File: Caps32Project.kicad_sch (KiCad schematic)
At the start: 23 parts, among them J1 Ph 2.0, J2 Sh 1.0, P1 USB_C_Plug_USB2.0, Q1 AO3401A, U1 MPU-6050, U2 MAX17048G_T10, U3 ESP32C3_SuperMini, U4 MCP73831-2-OT

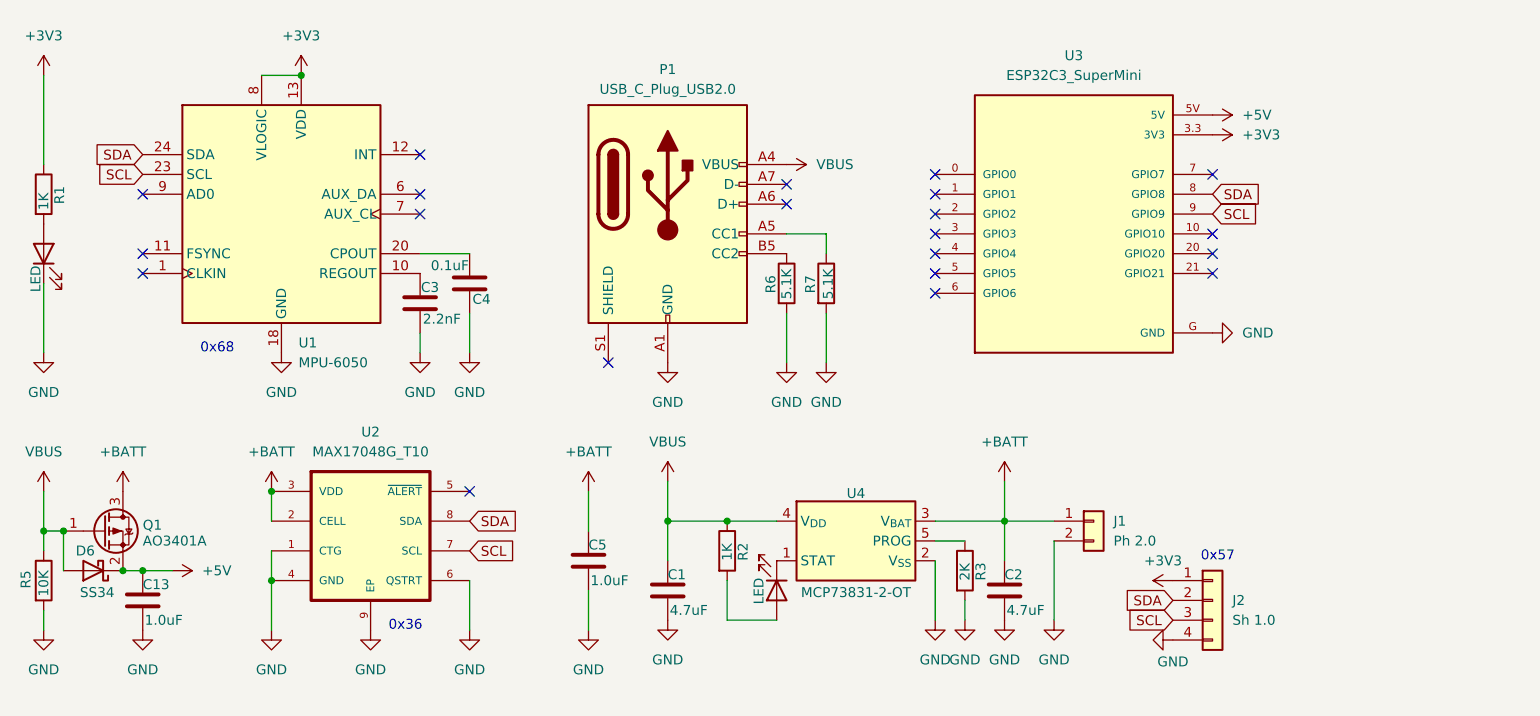
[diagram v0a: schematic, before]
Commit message: LGTM
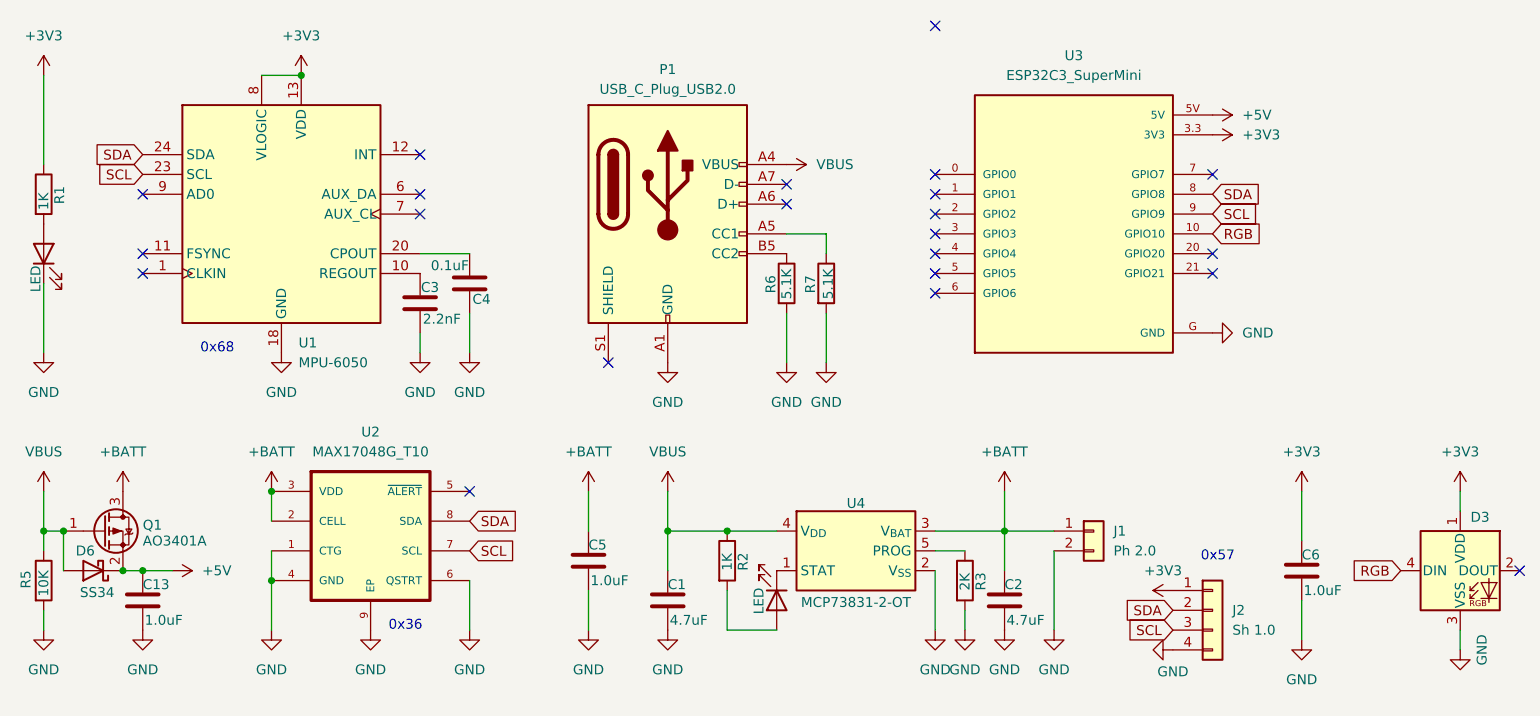
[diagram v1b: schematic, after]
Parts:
- added C6: 1.0uF, Capacitor_SMD:C_0402_1005Metric_Pad0.74x0.62mm_HandSolder, symbol Device:C
- added D3: WS2812B, LED_SMD:LED_WS2812B_PLCC4_5.0x5.0mm_P3.2mm, symbol LED:WS2812B
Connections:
- net +3V3: now also C6.1, D3.1 (VDD)
- net GND: now also C6.2, D3.3 (VSS)
- net RGB: now reaches U3.10 (GPIO10)
- net RGB: now also D3.4 (DIN)
- no-connect marks 21 -> 22
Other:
- moved on the sheet: C1, C2, J1, J2, R2, R3, U4

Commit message: MH42
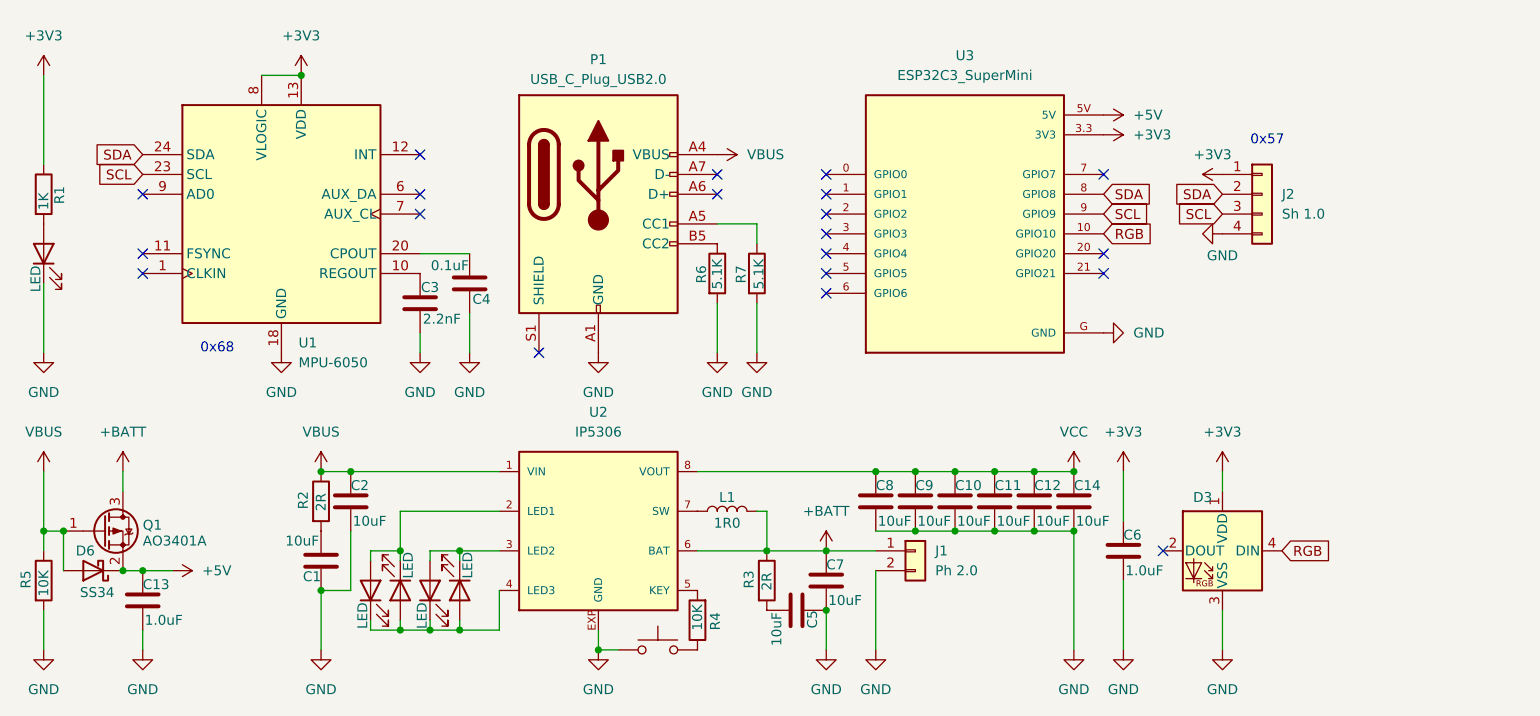
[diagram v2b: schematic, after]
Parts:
- removed U2: MAX17048G_T10, Custom:SON50P200X200X80-9N, symbol Custom:MAX17048G_T10
- removed U4: MCP73831-2-OT, Package_TO_SOT_SMD:SOT-23-5, symbol Battery_Management:MCP73831-5-OT
- added C10, C11, C12, C14, C7, C8, C9: 10uF, Capacitor_SMD:C_0402_1005Metric_Pad0.74x0.62mm_HandSolder, symbol Device:C
- added D4, D5, D7: LED, LED_SMD:LED_0402_1005Metric_Pad0.77x0.64mm_HandSolder, symbol Device:LED
- added L1: 1R0, symbol Device:L
- added R4: 10K, Resistor_SMD:R_0402_1005Metric_Pad0.72x0.64mm_HandSolder, symbol Device:R
- added SW1: SW_Push, symbol Switch:SW_Push
- added U2: IP5306, IP5306:SOP8-P, symbol Custom:IP5306
- C1, C2: value 4.7uF -> 10uF
- C5: value 1.0uF -> 10uF
- R2: value 1K -> 2R
- R3: value 2K -> 2R
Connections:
- net +BATT: now also R3.1, C7.1, L1.2, U2.6 (BAT); no longer C2.1, C5.1
- net GND: now also C1.1, C5.1, C10.2, C11.2, C12.2, C14.2, C7.2, C8.2, C9.2, SW1.1, U2.EXP (GND); no longer C1.2, C5.2, R3.2
- net VBUS: now also C2.1, U2.1 (VIN); no longer C1.1
- net at D2.2 (A): now also D4.1 (K), U2.2 (LED1); no longer R2.2
- net at D2.1 (K): now also D4.2 (A), D5.1 (K), D7.2 (A), U2.4 (LED3)
- new net: D5.2 (A), D7.1 (K), U2.3 (LED2)
- new net: C1.2, R2.2
- new net: C5.2, R3.2
- new net: R4.1, SW1.2
- new net: R4.2, U2.5 (KEY)
- new net: L1.1, U2.7 (SW)
- new net VCC: C10.1, C11.1, C12.1, C14.1, C8.1, C9.1, U2.8 (VOUT)
- no-connect marks 22 -> 20
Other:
- moved on the sheet: C6, D3, J1, J2, P1, R6, R7, U3

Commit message: Tweak
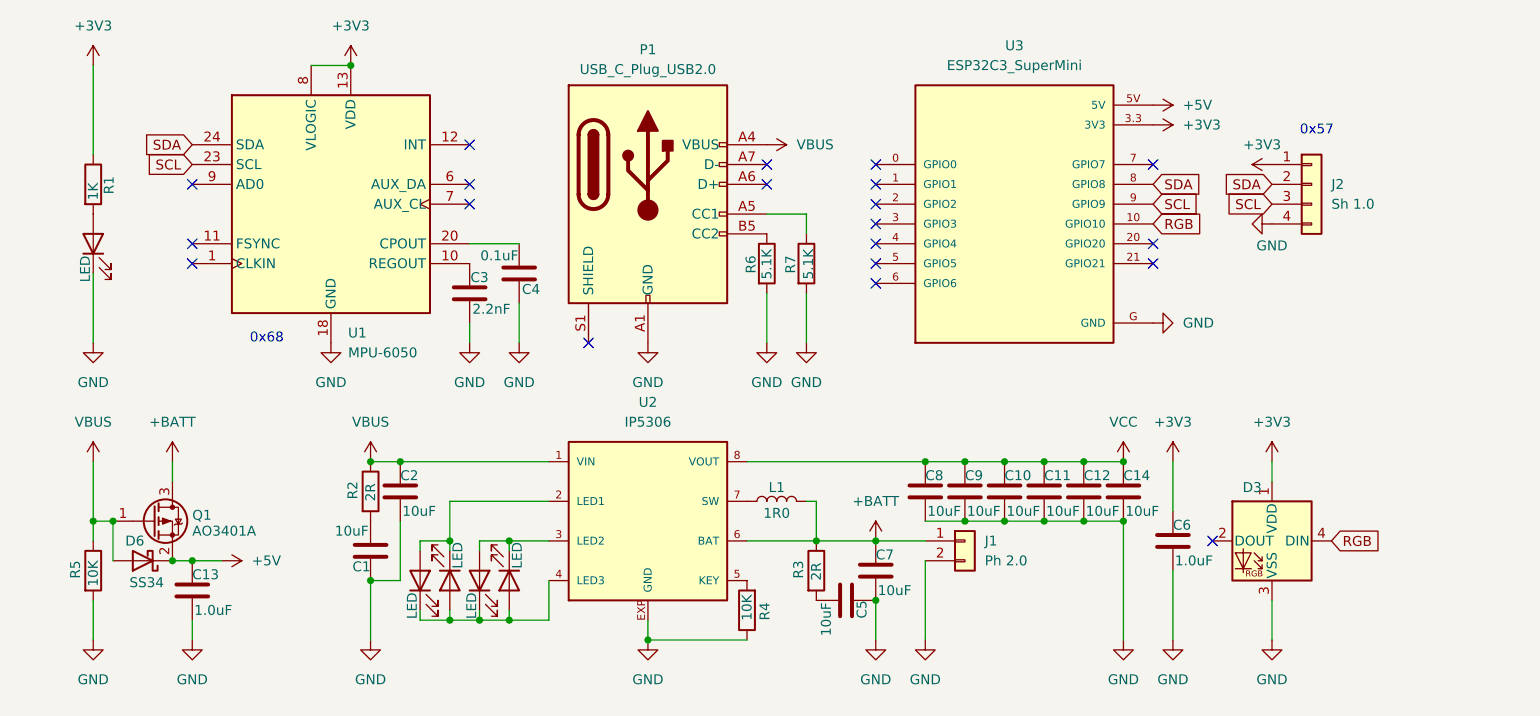
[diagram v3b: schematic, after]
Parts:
- removed SW1: SW_Push, symbol Switch:SW_Push
- L1: footprint (none) -> Inductor_SMD:L_6.3x6.3_H3
- P1: footprint Connector_USB:USB_C_Receptacle_XKB_U262-16XN-4BVC11 -> Connector_USB:USB_C_Receptacle_Palconn_UTC16-G
- U2: footprint IP5306:SOP8-P -> Custom:IP5306
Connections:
- net GND: now also R4.1
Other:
- moved on the sheet: C1, C10, C11, C12, C13, C14, C2, C3, C4, C5, C6, C7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

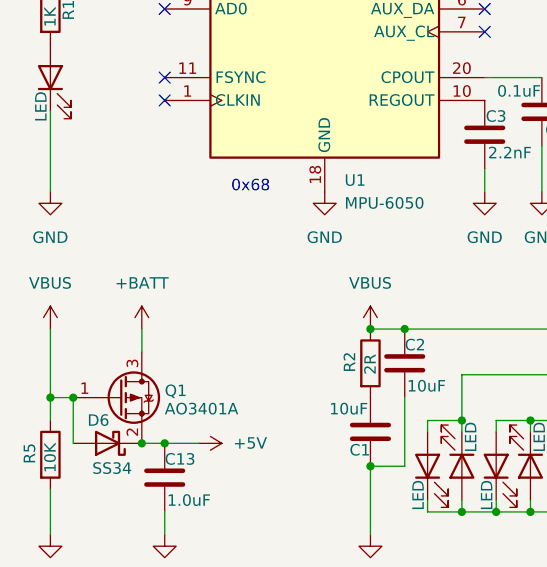
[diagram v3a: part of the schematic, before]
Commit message: Non Latch
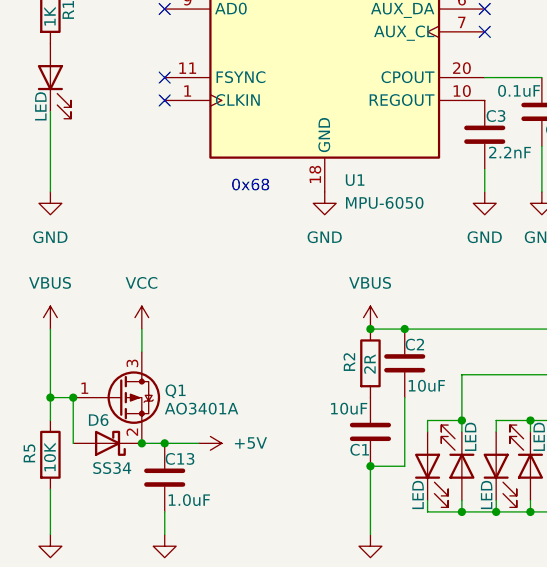
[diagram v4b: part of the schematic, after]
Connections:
- net +BATT: no longer Q1.3 (D)
- net VCC: now also Q1.3 (D)
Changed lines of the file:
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@@
+	)
+	(symbol
+		(lib_id "power:VCC")
+		(at 36.83 72.39 0)
+		(unit 1)
+		(exclude_from_sim no)
+		(in_bom yes)
+		(on_board yes)
+		(dnp no)
+		(fields_autoplaced yes)
+		(property "Reference" "#PWR022"
+			(at 36.83 76.2 0)
+			(effects
+				(font
+					(size 1.27 1.27)
+				)
+				(hide yes)
+			)
+		)
+		(property "Value" "VCC"
+			(at 36.83 67.31 0)
+			(effects
+				(font
+					(size 1.27 1.27)
+				)
+			)
+		)
+		(property "Footprint" ""
+			(at 36.83 72.39 0)
+			(effects
+				(font
+					(size 1.27 1.27)
+				)
+				(hide yes)
+			)
+		)
+		(property "Datasheet" ""
+			(at 36.83 72.39 0)
+			(effects
+				(font
+					(size 1.27 1.27)
+				)
+				(hide yes)
+			)
+		)
+		(property "Description" "Power symbol creates a global label with name \"VCC\""
+			(at 36.83 72.39 0)
+			(effects
+				(font
+					(size 1.27 1.27)
+				)
+				(hide yes)
+			)
+		)
+		(pin "1"
+		)
+		(instances
+			(project "Caps32Project"
+				(path "/c1972a26-8b03-42e6-af88-e08ef9733d83"
+					(reference "#PWR022")
+					(unit 1)
+				)
+			)
+		)
 	)
 	(symbol
@@
 					(unit 1)
 				)
-			)
-		)
-	)
-	(symbol
-		(lib_id "power:+BATT")
-		(at 36.83 72.39 0)
-		(unit 1)
-		(exclude_from_sim no)
-		(in_bom yes)
-		(on_board yes)
-		(dnp no)
-		(fields_autoplaced yes)
-		(property "Reference" "#PWR022"
-			(at 36.83 76.2 0)
-			(effects
-				(font
-					(size 1.27 1.27)
-				)
-				(hide yes)
-			)
-		)
-		(property "Value" "+BATT"
-			(at 36.83 67.31 0)
-			(effects
-				(font
-					(size 1.27 1.27)
-				)
-			)
-		)
-		(property "Footprint" ""
-			(at 36.83 72.39 0)
-			(effects
-				(font
-					(size 1.27 1.27)
-				)
-				(hide yes)
-			)
-		)
-		(property "Datasheet" ""
-			(at 36.83 72.39 0)
-			(effects
-				(font
-					(size 1.27 1.27)
-				)
-				(hide yes)
-			)
-		)
-		(property "Description" "Power symbol creates a global label with name \"+BATT\""
-			(at 36.83 72.39 0)
-			(effects
-				(font
-					(size 1.27 1.27)
-				)
-				(hide yes)
-			)
-		)
-		(pin "1"
-		)
-		(instances
-			(project "Caps"
-				(path "/c1972a26-8b03-42e6-af88-e08ef9733d83"
-					(reference "#PWR022")
-					(unit 1)
-				)

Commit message: Tweak
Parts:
- U3: footprint Custom:ESP32C3_Supermini_THT -> Custom:Supermini_Custom
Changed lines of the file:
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@@
 			)
 		)
-		(property "Footprint" "Custom:ESP32C3_Supermini_THT"
+		(property "Footprint" "Custom:Supermini_Custom"
 			(at 144.78 39.37 0)
 			(effects

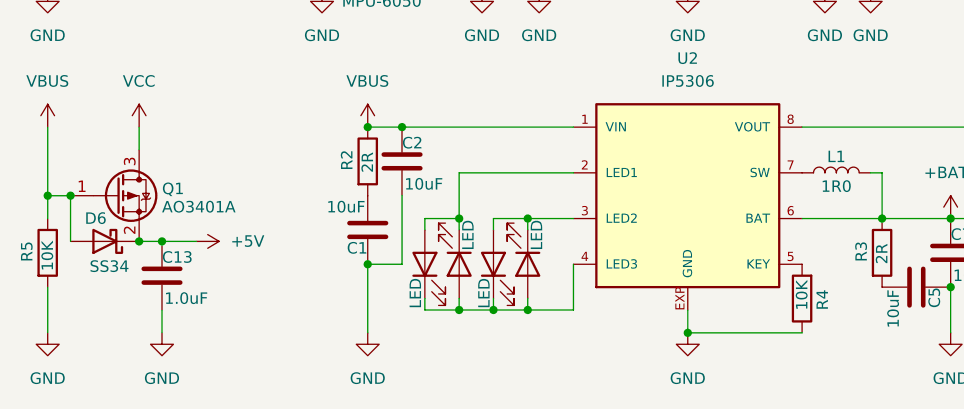
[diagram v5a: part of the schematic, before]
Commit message: Fixing
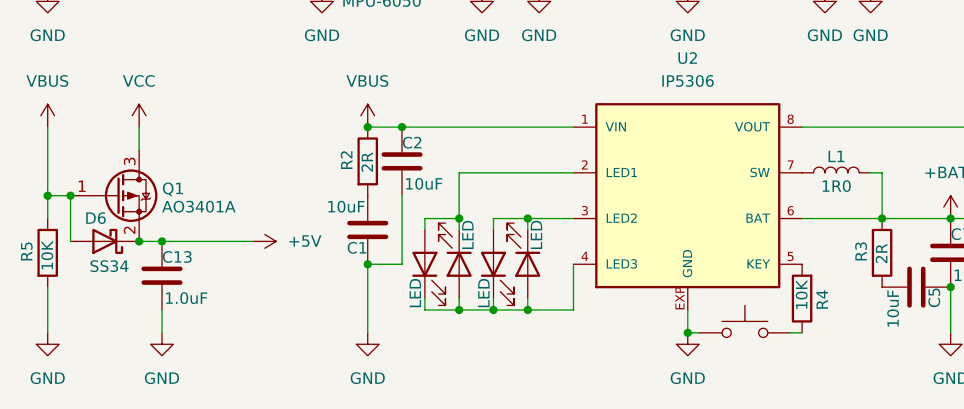
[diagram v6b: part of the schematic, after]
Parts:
- added SW1: SW_Push, Button_Switch_SMD:SW_Push_1TS009xxxx-xxxx-xxxx_6x6x5mm, symbol Switch:SW_Push
- J1: footprint Connector_JST:JST_PH_S2B-PH-K_1x02_P2.00mm_Horizontal -> Connector_JST:JST_PH_S2B-PH-SM4-TB_1x02-1MP_P2.00mm_Horizontal
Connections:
- net GND: now also SW1.1; no longer R4.1
- new net: R4.1, SW1.2
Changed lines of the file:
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@@
 	)
 	(junction
-		(at 97.79 95.25)
-		(diameter 0)
-		(color 0 0 0 0)
-	)
-	(junction
 		(at 127 90.17)
 		(diameter 0)
@@
 	)
 	(junction
+		(at 97.79 95.25)
+		(diameter 0)
+		(color 0 0 0 0)
+	)
+	(junction
 		(at 26.67 80.01)
 		(diameter 0)
@@
 	(wire
 		(pts
+			(xy 97.79 95.25) (xy 99.06 95.25)
+		)
+		(stroke
+			(width 0)
+			(type default)
+		)
+	)
+	(wire
+		(pts
 			(xy 118.11 40.64) (xy 113.03 40.64)
 		)
@@
 	(wire
 		(pts
-			(xy 97.79 95.25) (xy 110.49 95.25)
+			(xy 109.22 95.25) (xy 110.49 95.25)
 		)
 		(stroke
@@
 	(wire
 		(pts
-			(xy 43.18 85.09) (xy 39.37 85.09)
+			(xy 49.53 85.09) (xy 39.37 85.09)
 		)
 		(stroke
@@
 	(symbol
 		(lib_id "power:+5V")
-		(at 43.18 85.09 270)
+		(at 49.53 85.09 270)
 		(unit 1)
 		(exclude_from_sim no)
@@
 		(fields_autoplaced yes)
 		(property "Reference" "#PWR014"
-			(at 39.37 85.09 0)
+			(at 45.72 85.09 0)
 			(effects
 				(font
@@
 		)
 		(property "Value" "+5V"
-			(at 46.99 85.0899 90)
+			(at 53.34 85.0899 90)
 			(effects
 				(font
@@
 		)
 		(property "Footprint" ""
-			(at 43.18 85.09 0)
+			(at 49.53 85.09 0)
 			(effects
 				(font
@@
 		)
 		(property "Datasheet" ""
-			(at 43.18 85.09 0)
+			(at 49.53 85.09 0)
 			(effects
 				(font
@@
 		)
 		(property "Description" "Power symbol creates a global label with name \"+5V\""
-			(at 43.18 85.09 0)
+			(at 49.53 85.09 0)
 			(effects
 				(font
@@
 	)
 	(symbol
+		(lib_id "Switch:SW_Push")
+		(at 104.14 95.25 0)
+		(unit 1)
+		(exclude_from_sim no)
+		(in_bom yes)
+		(on_board yes)
+		(dnp no)
+		(fields_autoplaced yes)
+		(property "Reference" "SW1"
+			(at 104.14 87.63 0)
+			(effects
+				(font
+					(size 1.27 1.27)
+				)
+				(hide yes)
+			)
+		)
+		(property "Value" "SW_Push"
+			(at 104.14 90.17 0)
+			(effects
+				(font
+					(size 1.27 1.27)
+				)
+				(hide yes)
+			)
+		)
+		(property "Footprint" "Button_Switch_SMD:SW_Push_1TS009xxxx-xxxx-xxxx_6x6x5mm"
+			(at 104.14 90.17 0)
+			(effects
+				(font
+					(size 1.27 1.27)
+				)
+				(hide yes)
+			)
+		)
+		(property "Datasheet" "~"
+			(at 104.14 90.17 0)
+			(effects
+				(font
+					(size 1.27 1.27)
+				)
+				(hide yes)
+			)
+		)
+		(property "Description" "Push button switch, generic, two pins"
+			(at 104.14 95.25 0)
+			(effects
+				(font
+					(size 1.27 1.27)
+				)
+				(hide yes)
+			)
+		)
+		(pin "1"
+		)
+		(pin "2"
+		)
+		(instances
+			(project ""
+				(path "/c1972a26-8b03-42e6-af88-e08ef9733d83"
+					(reference "SW1")
+					(unit 1)
+				)
+			)
+		)
+	)
+	(symbol
 		(lib_id "Device:L")
 		(at 114.3 77.47 90)
@@
 			)
 		)
-		(property "Footprint" "Connector_JST:JST_PH_S2B-PH-K_1x02_P2.00mm_Horizontal"
+		(property "Footprint" "Connector_JST:JST_PH_S2B-PH-SM4-TB_1x02-1MP_P2.00mm_Horizontal"
 			(at 138.43 82.55 0)
 			(effects
